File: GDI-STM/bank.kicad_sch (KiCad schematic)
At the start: 23 parts, among them Q19 BUK9230-100B, Q20 BUK9230-100B, Q21 BUK9230-100B, Q22 BUK9230-100B

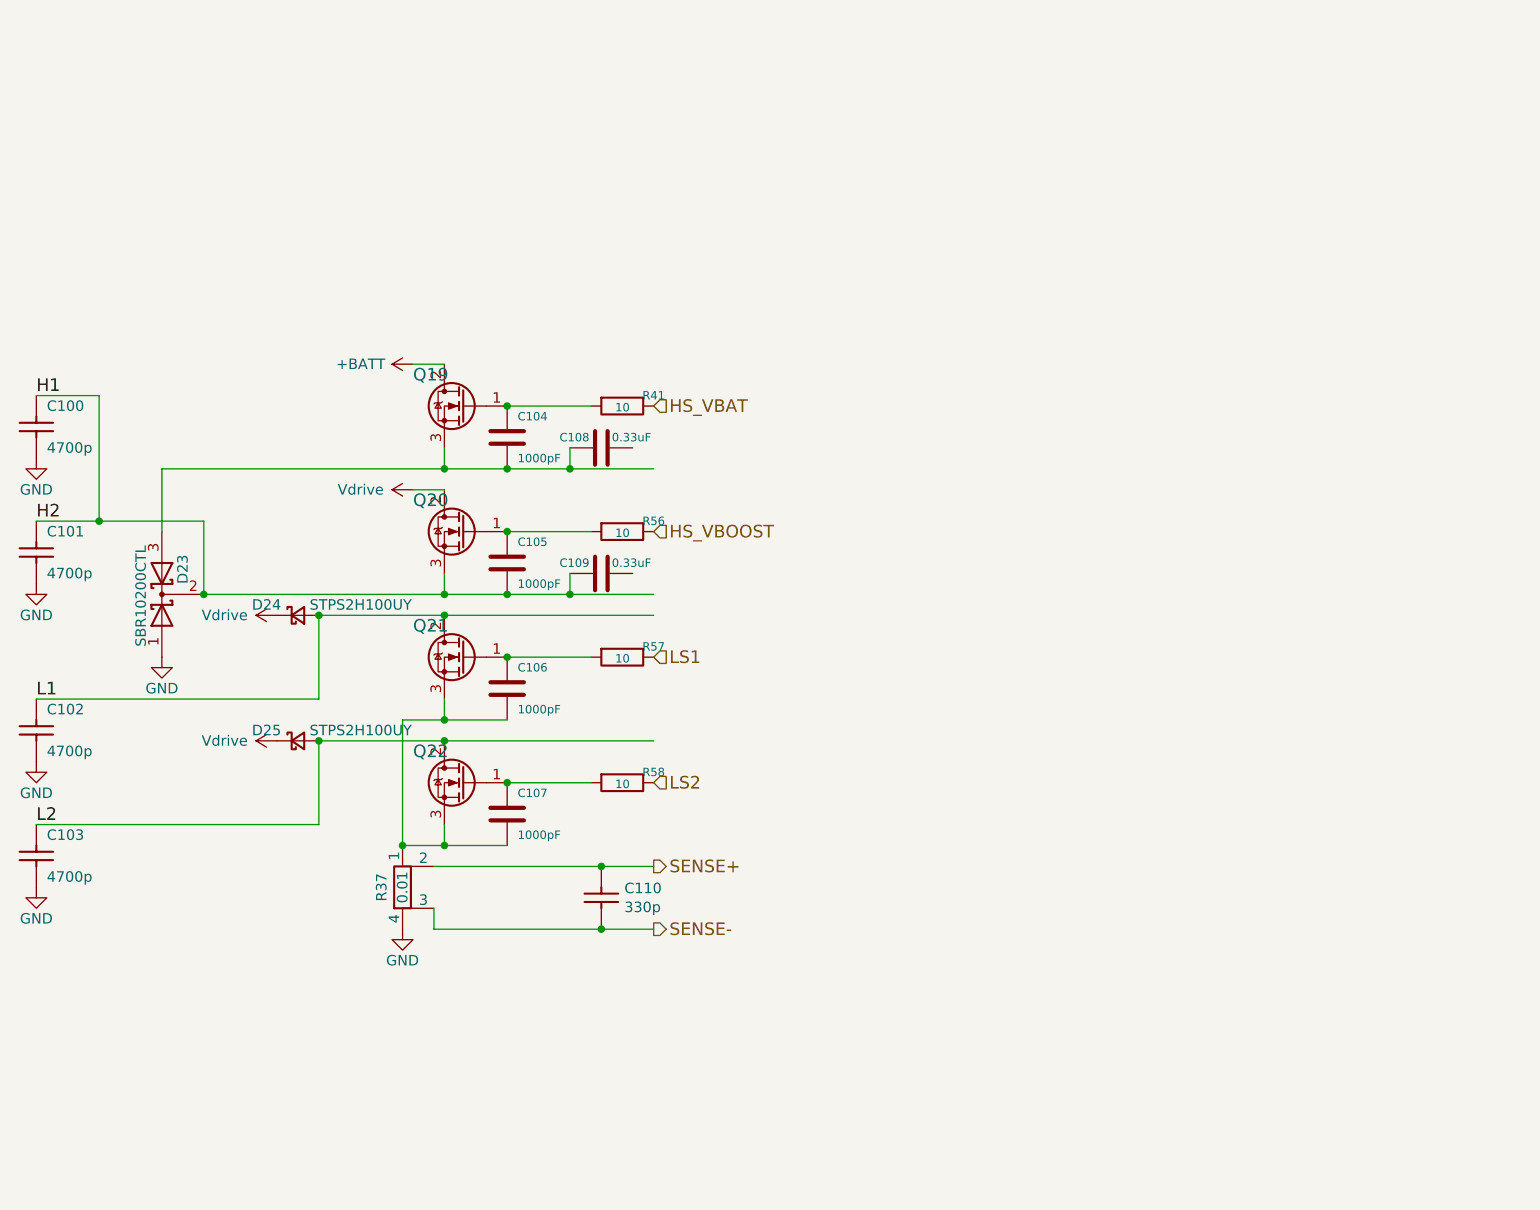
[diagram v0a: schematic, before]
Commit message: Upd SCH
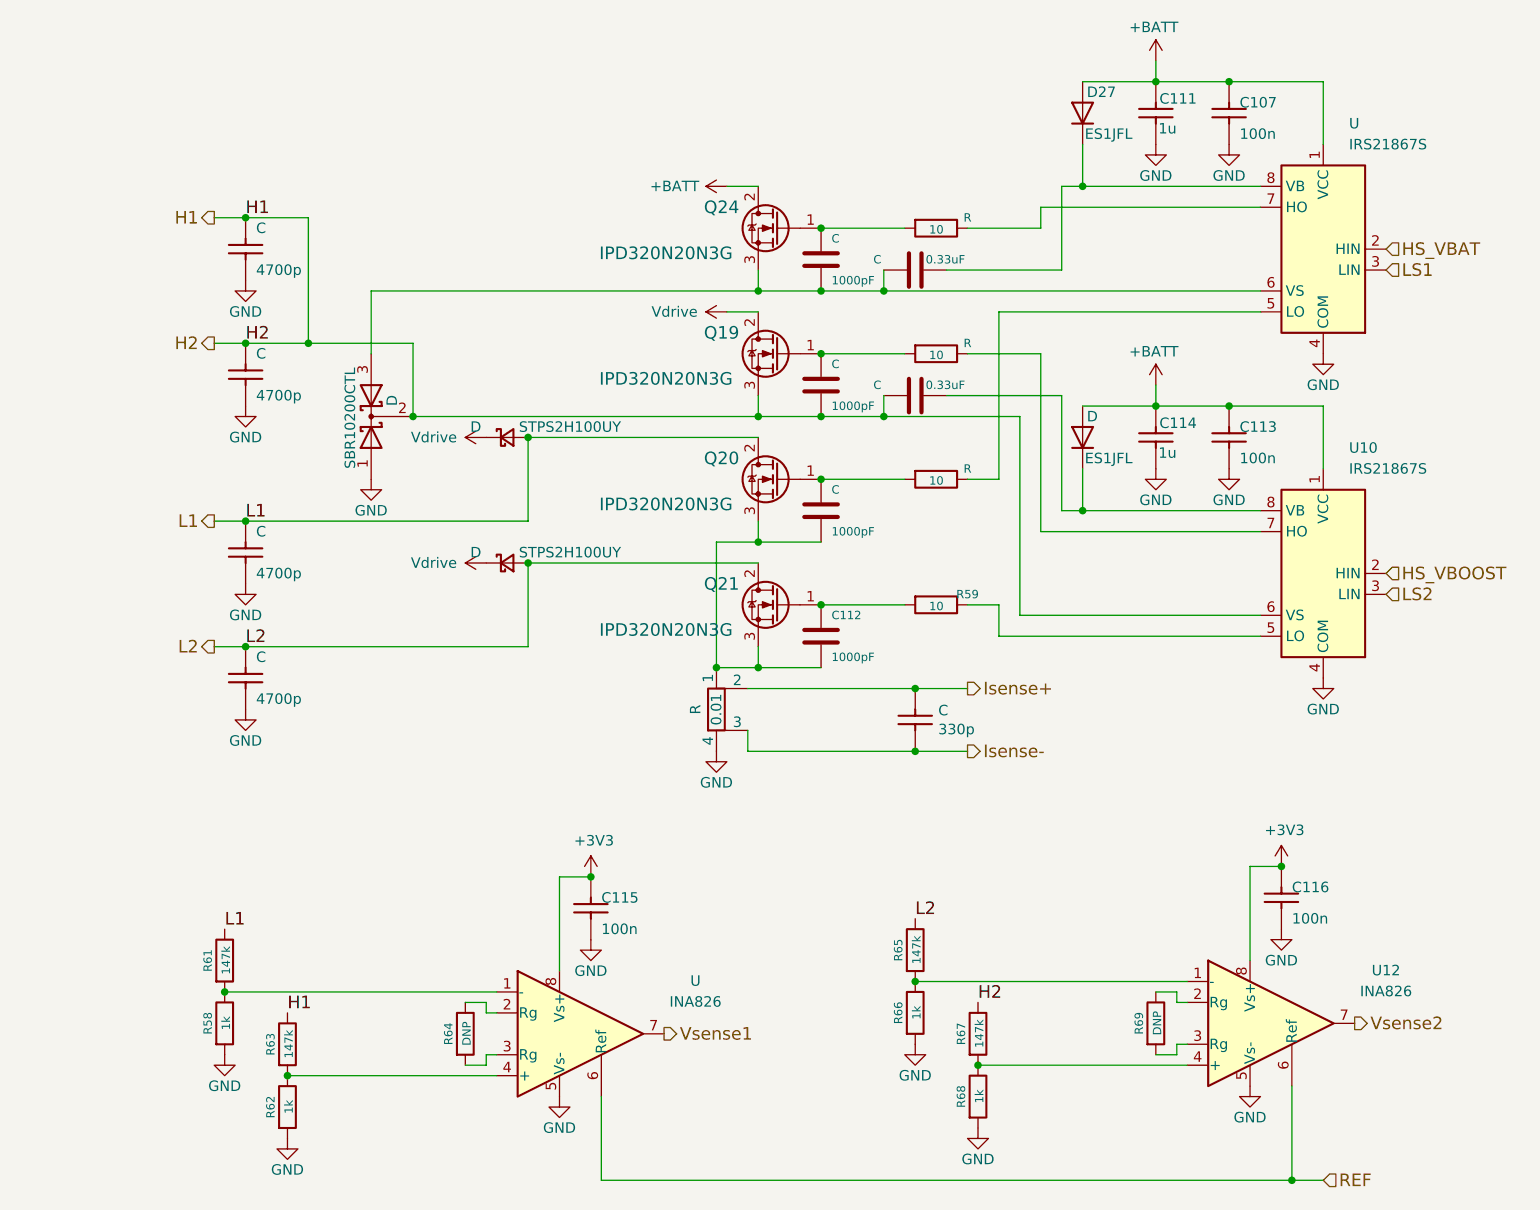
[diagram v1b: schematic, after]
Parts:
- removed C107: 1000pF, Capacitor_SMD:C_0603_1608Metric, symbol Device:C
- removed Q22: BUK9230-100B, Package_TO_SOT_SMD:TO-252-2, symbol Device:Q_NMOS_GDS
- added C107, C113, C115, C116: 100n, hellen-one-common:C0603, symbol hellen-one-common:Cap
- added C111, C114: 1u, hellen-one-common:C0603, symbol hellen-one-common:Cap
- added C112: 1000pF, Capacitor_SMD:C_0603_1608Metric, symbol Device:C
- added D, D27: ES1JFL, Diode_SMD:D_SOD-123F, symbol Device:D
- added Q24: IPD320N20N3G, Package_TO_SOT_SMD:TO-252-2, symbol Device:Q_NMOS_GDS
- added R59: 10, Resistor_SMD:R_0603_1608Metric, symbol Device:R
- added R61, R63, R65, R67: 147k, Resistor_SMD:R_0603_1608Metric, symbol Device:R
- added R62, R66, R68: 1k, Resistor_SMD:R_0603_1608Metric, symbol Device:R
- added R64, R69: DNP, Resistor_SMD:R_0603_1608Metric, symbol Device:R
- added U, U10: IRS21867S, Package_SO:SOIC-8_3.9x4.9mm_P1.27mm, symbol Driver_FET:IRS21867S
- added U, U12: INA826, Package_SO:SOIC-8_3.9x4.9mm_P1.27mm, symbol Amplifier_Instrumentation:INA821xD
- Q19, Q20, Q21: value BUK9230-100B -> IPD320N20N3G; LCSC C89735 -> C501515; MFG,MFG# Nexperia,BUK9230-100B -> (none); VEND1,VEND1# DIGI,1727-4708-1-ND -> (none); VEND2,VEND2# , -> (none)
- R58: value 10 -> 1k; LCSC C22859 -> C21190
- renumbered C105 to C, C108 to C, C102 to C, C101 to C, C104 to C, C103 to C, C106 to C, C109 to C, C110 to C, C100 to C, D24 to D, D25 to D, D23 to D, R57 to R, R41 to R, R56 to R, R37 to R
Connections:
- net +BATT: now also C107.2, C111.2, C113.2, C114.2, D.2 (A), D27.2 (A), Q24.2 (D), U.1 (VCC), U10.1 (VCC); no longer Q19.2 (D)
- net GND: now also R58.2, C107.1, C111.1, C113.1, C114.1, C115.1, C116.1, R62.2, R66.2, R68.2, U.4 (COM), U.5 (Vs-), U10.4 (COM), U12.5 (Vs-)
- net H1: now also Q19.3 (S), R63.1, R67.1, U10.6 (VS); no longer Q20.3 (S)
- net HS_VBAT: now also U.2 (HIN); no longer R.1
- net HS_VBOOST: now also U10.2 (HIN); no longer R.1
- net L1: now also Q20.2 (D), R61.1; no longer Q21.2 (D)
- net L2: now also Q21.2 (D), R65.1
- net LS1: now also U.3 (LIN); no longer R.1
- net LS2: now also U10.3 (LIN); no longer R58.1
- net Vdrive: now also Q19.2 (D); no longer Q20.2 (D)
- net at C.2, R.2: now also Q19.1 (G); no longer Q20.1 (G)
- net at C.1, Q21.3 (S), R.1: now also Q20.3 (S), C112.1
- net at C.2, R.2: now also Q20.1 (G); no longer Q21.1 (G)
- net at C.1: now also D27.1 (K), U.8 (VB)
- net at C.1, C.2, D.3 (A): now also Q24.3 (S), U.6 (VS); no longer Q19.3 (S)
- net at C.2, R.2: now also Q24.1 (G); no longer Q19.1 (G)
- net at C.1: now also D.1 (K), U10.8 (VB)
- net SENSE+ renamed Isense+
- net SENSE- renamed Isense-
- new net: R58.1, R61.2, U.1 (-)
- new net: R.1, U.5 (LO)
- new net: C112.2, Q21.1 (G), R59.2
- new net: R.1, U.7 (HO)
- new net: R65.2, R66.1, U12.1 (-)
- new net: R67.2, R68.1, U12.4 (+)
- new net: R69.1, U12.2 (Rg)
- new net: R69.2, U12.3 (Rg)
- new net: R62.1, R63.2, U.4 (+)
- new net: R.1, U10.7 (HO)
- new net: R59.1, U10.5 (LO)
- new net: R64.1, U.2 (Rg)
- new net: R64.2, U.3 (Rg)
- new net +3V3: C115.2, C116.2, U.8 (Vs+), U12.8 (Vs+)
- new net REF: U.6 (Ref), U12.6 (Ref)
- new net Vsense1: U.7
- new net Vsense2: U12.7
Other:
- moved on the sheet: C, D, R
